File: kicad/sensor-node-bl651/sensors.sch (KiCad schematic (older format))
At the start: 11 parts, among them M1 MMC5603NJ, M2 MXC4005XC, U3 LSM303AGR

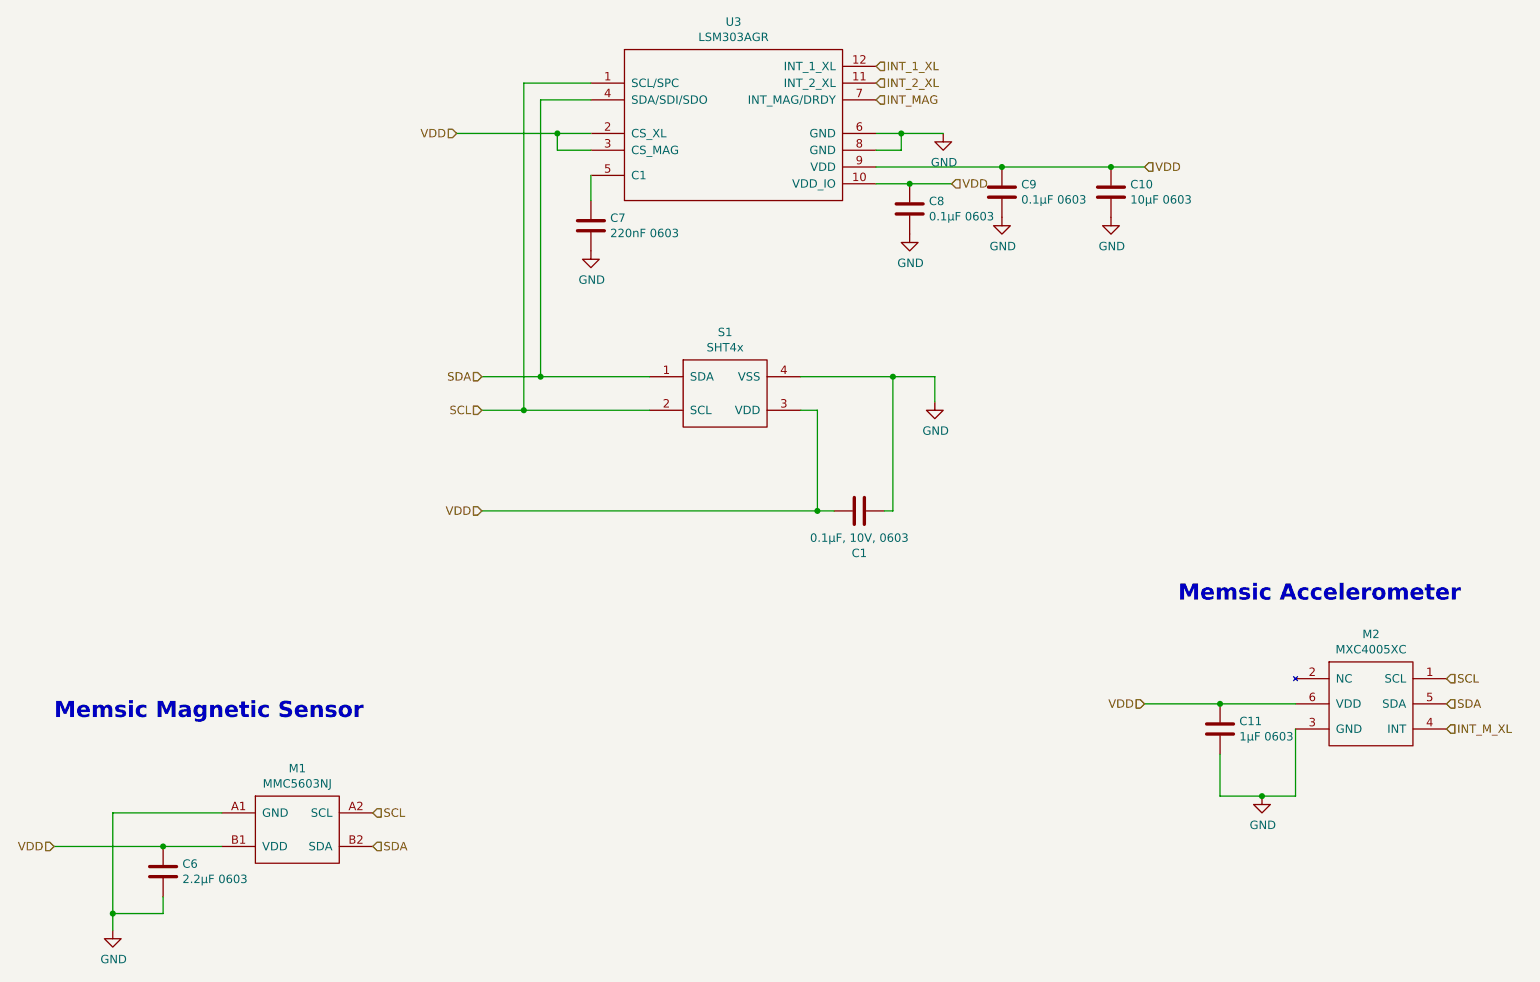
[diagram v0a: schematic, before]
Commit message: remove memsic sensors
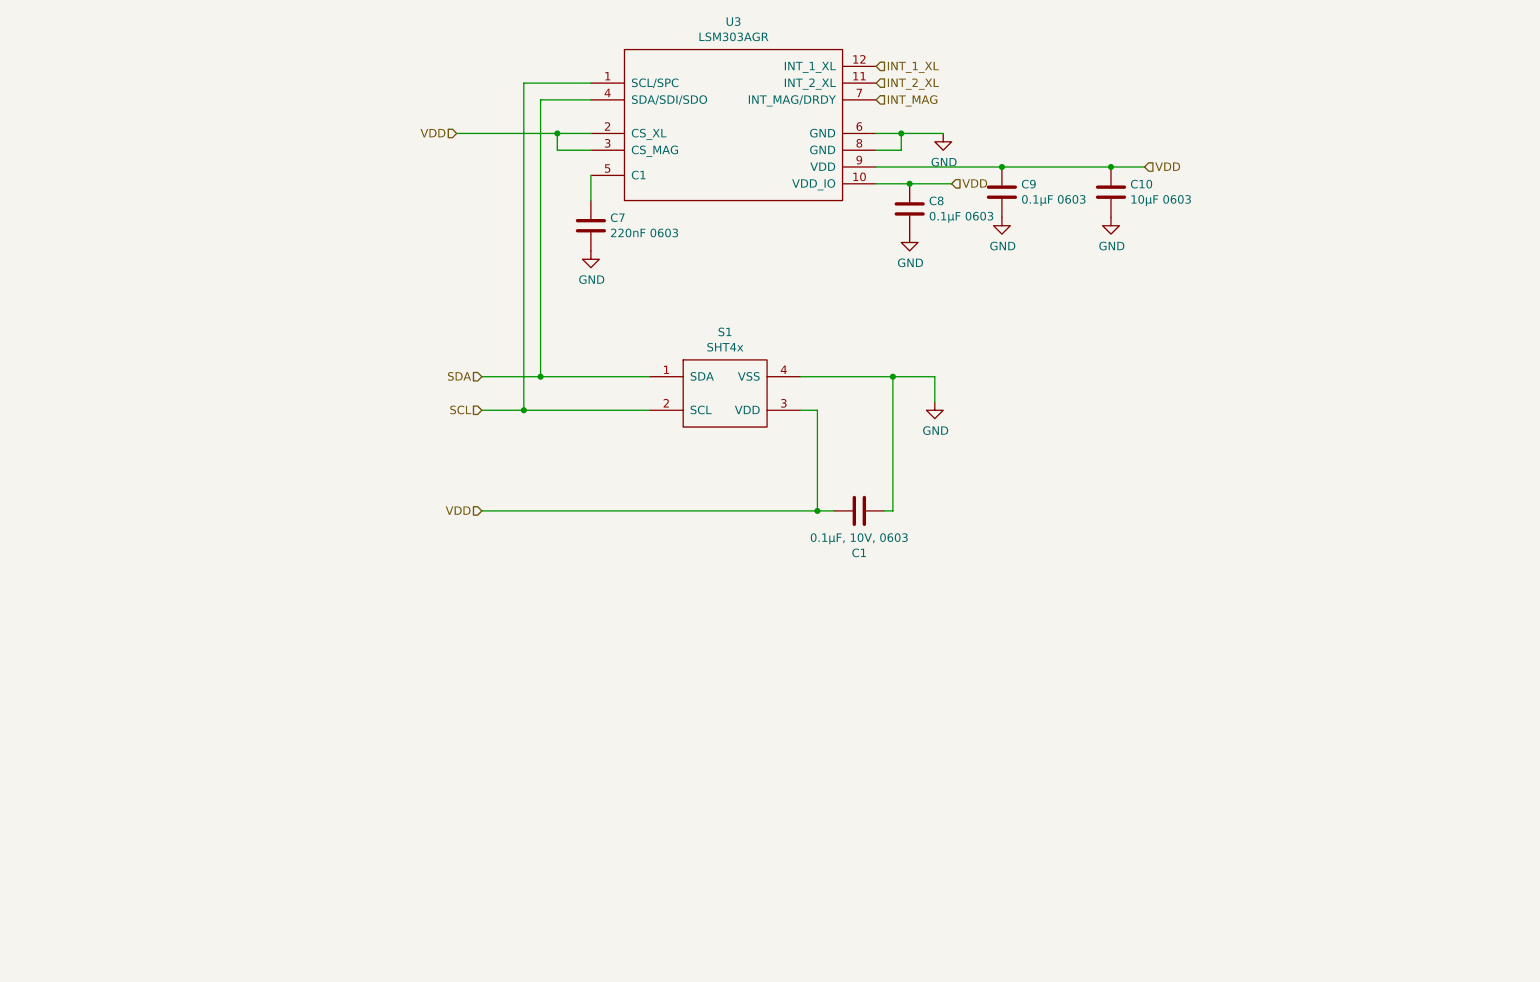
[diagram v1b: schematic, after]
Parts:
- removed C11: 1µF 0603, Capacitor_SMD:C_0603_1608Metric, symbol Device:C
- removed C6: 2.2µF 0603, Capacitor_SMD:C_0603_1608Metric, symbol Device:C
- removed M1: MMC5603NJ, HH_Memsic:MMC5603NJ, symbol HH_Memsic:MMC5603NJ
- removed M2: MXC4005XC, HH_Memsic:MXC400xXC, symbol HH_Memsic:MXC4005XC
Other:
- note removed: "Memsic Accelerometer"
- note removed: "Memsic Magnetic Sensor"
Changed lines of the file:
@@
 Wire Wire Line
 	4850 3400 5500 3400
-$Comp
-L HH_Memsic:MXC4005XC M2
-U 1 1 60BA1560
-P 9800 5350
-F 0 "M2" H 9800 5765 50  0000 C CNN
-F 1 "MXC4005XC" H 9800 5674 50  0000 C CNN
-F 2 "HH_Memsic:MXC400xXC" H 9800 5350 50  0001 C CNN
-F 3 "https://media.digikey.com/pdf/Data%20Sheets/MEMSIC%20PDFs/MXC400xXC_Rev.B_4-24-15.pdf" H 9800 5350 50  0001 C CNN
-F 4 "1267-1075-1-ND" H 9800 5350 50  0001 C CNN "Digi-Key Part Number"
-F 5 "Memsic Inc." H 9800 5350 50  0001 C CNN "Manufacturer"
-F 6 "MXC4005XC" H 9800 5350 50  0001 C CNN "Manufacturer Part Number"
-F 7 "THREE AXIS ACCELEROMETER" H 9800 5350 50  0001 C CNN "Description"
-	1    9800 5350
-	1    0    0    -1
-$EndComp
-$Comp
-L Device:C C11
-U 1 1 60BA9A12
-P 8900 5500
-F 0 "C11" H 9015 5546 50  0000 L CNN
-F 1 "1µF 0603" H 9015 5455 50  0000 L CNN
-F 2 "Capacitor_SMD:C_0603_1608Metric" H 8938 5350 50  0001 C CNN
-F 3 "~" H 8900 5500 50  0001 C CNN
-	1    8900 5500
-	1    0    0    -1
-$EndComp
-Wire Wire Line
-	8900 5350 9350 5350
-Wire Wire Line
-	9350 5500 9350 5900
-Wire Wire Line
-	9350 5900 9150 5900
-Wire Wire Line
-	8900 5900 8900 5650
-$Comp
-L power:GND #PWR010
-U 1 1 60BABF47
-P 9150 5900
-F 0 "#PWR010" H 9150 5650 50  0001 C CNN
-F 1 "GND" H 9155 5727 50  0000 C CNN
-F 2 "" H 9150 5900 50  0001 C CNN
-F 3 "" H 9150 5900 50  0001 C CNN
-	1    9150 5900
-	1    0    0    -1
-$EndComp
-Connection ~ 9150 5900
-Wire Wire Line
-	9150 5900 8900 5900
-Text HLabel 8450 5350 0    50   Input ~ 0
-VDD
-Wire Wire Line
-	8900 5350 8450 5350
-Connection ~ 8900 5350
-Text HLabel 10250 5350 2    50   Input ~ 0
-SDA
-Text HLabel 10250 5200 2    50   Input ~ 0
-SCL
-Text HLabel 10250 5500 2    50   Input ~ 0
-INT_M_XL
-Text Notes 8650 4750 0    96   ~ 19
-Memsic Accelerometer
-$Comp
-L HH_Memsic:MMC5603NJ M1
-U 1 1 60BAED17
-P 3400 6100
-F 0 "M1" H 3400 6465 50  0000 C CNN
-F 1 "MMC5603NJ" H 3400 6374 50  0000 C CNN
-F 2 "HH_Memsic:MMC5603NJ" H 3400 6100 50  0001 C CNN
-F 3 "https://media.digikey.com/pdf/Data%20Sheets/MEMSIC%20PDFs/MMC5603NJ_RevB_7-12-18.pdf" H 3400 6100 50  0001 C CNN
-F 4 "1267-MMC5603NJCT-ND" H 3400 6100 50  0001 C CNN "Digi-Key Part Number"
-F 5 "Memsic Inc." H 3400 6100 50  0001 C CNN "Manufacturer"
-F 6 "MMC5603NJ" H 3400 6100 50  0001 C CNN "Manufacturer Part Number"
-F 7 "3-AXIS AMR MAGNETIC SENSOR" H 3400 6100 50  0001 C CNN "Description"
-	1    3400 6100
-	1    0    0    -1
-$EndComp
-Text Notes 1950 5450 0    96   ~ 19
-Memsic Magnetic Sensor
-$Comp
-L Device:C C6
-U 1 1 60BB6732
-P 2600 6350
-F 0 "C6" H 2715 6396 50  0000 L CNN
-F 1 "2.2µF 0603" H 2715 6305 50  0000 L CNN
-F 2 "Capacitor_SMD:C_0603_1608Metric" H 2638 6200 50  0001 C CNN
-F 3 "~" H 2600 6350 50  0001 C CNN
-	1    2600 6350
-	1    0    0    -1
-$EndComp
-$Comp
-L power:GND #PWR09
-U 1 1 60BB7121
-P 2300 6700
-F 0 "#PWR09" H 2300 6450 50  0001 C CNN
-F 1 "GND" H 2305 6527 50  0000 C CNN
-F 2 "" H 2300 6700 50  0001 C CNN
-F 3 "" H 2300 6700 50  0001 C CNN
-	1    2300 6700
-	1    0    0    -1
-$EndComp
-Wire Wire Line
-	2300 6700 2300 6600
-Wire Wire Line
-	2300 6000 2950 6000
-Wire Wire Line
-	2600 6500 2600 6600
-Wire Wire Line
-	2600 6600 2300 6600
-Connection ~ 2300 6600
-Wire Wire Line
-	2300 6600 2300 6000
-Text HLabel 1950 6200 0    50   Input ~ 0
-VDD
-Wire Wire Line
-	1950 6200 2600 6200
-Connection ~ 2600 6200
-Wire Wire Line
-	2600 6200 2950 6200
-Text HLabel 3850 6000 2    50   Input ~ 0
-SCL
-Text HLabel 3850 6200 2    50   Input ~ 0
-SDA
 $EndSCHEMATC

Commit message: add more sensors
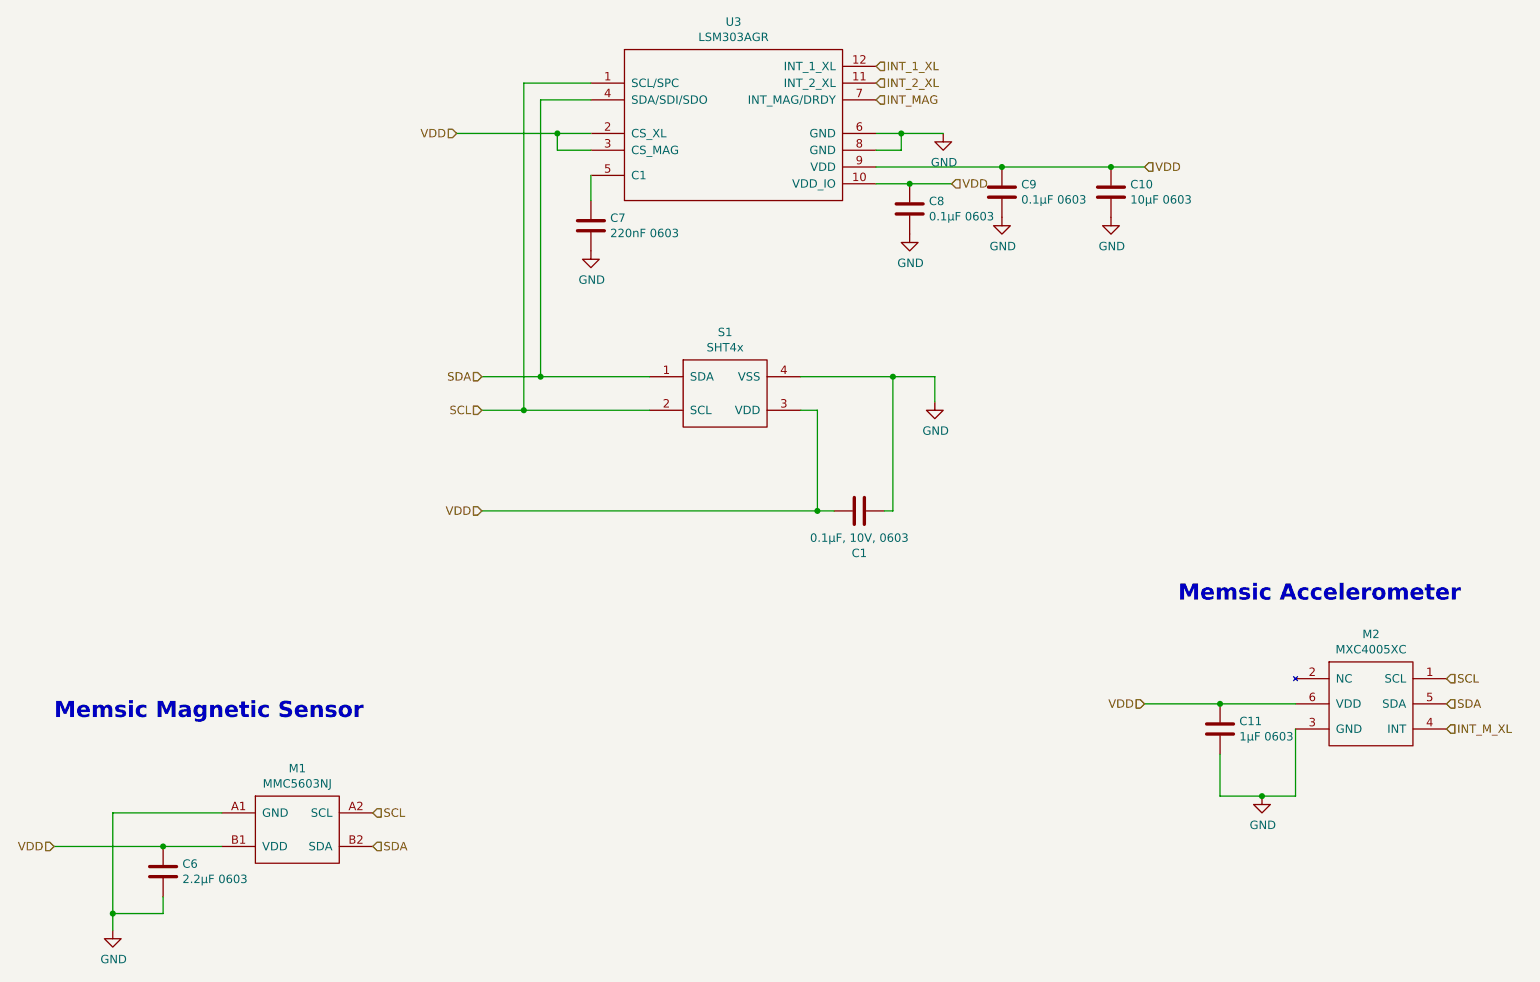
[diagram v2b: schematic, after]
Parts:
- added C11: 1µF 0603, Capacitor_SMD:C_0603_1608Metric, symbol Device:C
- added C6: 2.2µF 0603, Capacitor_SMD:C_0603_1608Metric, symbol Device:C
- added M1: MMC5603NJ, HH_Memsic:MMC5603NJ, symbol HH_Memsic:MMC5603NJ
- added M2: MXC4005XC, HH_Memsic:MXC400xXC, symbol HH_Memsic:MXC4005XC
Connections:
- net GND: now also C11.2, C6.2, M1.A1 (GND), M2.3 (GND)
- net SCL: now also M1.A2 (SCL), M2.1 (SCL)
- net SDA: now also M1.B2 (SDA), M2.5 (SDA)
- net VDD: now also C11.1, C6.1, M1.B1 (VDD), M2.6 (VDD)
- new net INT_M_XL: M2.4 (INT)
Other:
- note added: "Memsic Accelerometer"
- note added: "Memsic Magnetic Sensor"
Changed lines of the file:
@@
 Wire Wire Line
 	4850 3400 5500 3400
+$Comp
+L HH_Memsic:MXC4005XC M2
+U 1 1 60BA1560
+P 9800 5350
+F 0 "M2" H 9800 5765 50  0000 C CNN
+F 1 "MXC4005XC" H 9800 5674 50  0000 C CNN
+F 2 "HH_Memsic:MXC400xXC" H 9800 5350 50  0001 C CNN
+F 3 "https://media.digikey.com/pdf/Data%20Sheets/MEMSIC%20PDFs/MXC400xXC_Rev.B_4-24-15.pdf" H 9800 5350 50  0001 C CNN
+F 4 "1267-1075-1-ND" H 9800 5350 50  0001 C CNN "Digi-Key Part Number"
+F 5 "Memsic Inc." H 9800 5350 50  0001 C CNN "Manufacturer"
+F 6 "MXC4005XC" H 9800 5350 50  0001 C CNN "Manufacturer Part Number"
+F 7 "THREE AXIS ACCELEROMETER" H 9800 5350 50  0001 C CNN "Description"
+	1    9800 5350
+	1    0    0    -1
+$EndComp
+$Comp
+L Device:C C11
+U 1 1 60BA9A12
+P 8900 5500
+F 0 "C11" H 9015 5546 50  0000 L CNN
+F 1 "1µF 0603" H 9015 5455 50  0000 L CNN
+F 2 "Capacitor_SMD:C_0603_1608Metric" H 8938 5350 50  0001 C CNN
+F 3 "~" H 8900 5500 50  0001 C CNN
+	1    8900 5500
+	1    0    0    -1
+$EndComp
+Wire Wire Line
+	8900 5350 9350 5350
+Wire Wire Line
+	9350 5500 9350 5900
+Wire Wire Line
+	9350 5900 9150 5900
+Wire Wire Line
+	8900 5900 8900 5650
+$Comp
+L power:GND #PWR010
+U 1 1 60BABF47
+P 9150 5900
+F 0 "#PWR010" H 9150 5650 50  0001 C CNN
+F 1 "GND" H 9155 5727 50  0000 C CNN
+F 2 "" H 9150 5900 50  0001 C CNN
+F 3 "" H 9150 5900 50  0001 C CNN
+	1    9150 5900
+	1    0    0    -1
+$EndComp
+Connection ~ 9150 5900
+Wire Wire Line
+	9150 5900 8900 5900
+Text HLabel 8450 5350 0    50   Input ~ 0
+VDD
+Wire Wire Line
+	8900 5350 8450 5350
+Connection ~ 8900 5350
+Text HLabel 10250 5350 2    50   Input ~ 0
+SDA
+Text HLabel 10250 5200 2    50   Input ~ 0
+SCL
+Text HLabel 10250 5500 2    50   Input ~ 0
+INT_M_XL
+Text Notes 8650 4750 0    96   ~ 19
+Memsic Accelerometer
+$Comp
+L HH_Memsic:MMC5603NJ M1
+U 1 1 60BAED17
+P 3400 6100
+F 0 "M1" H 3400 6465 50  0000 C CNN
+F 1 "MMC5603NJ" H 3400 6374 50  0000 C CNN
+F 2 "HH_Memsic:MMC5603NJ" H 3400 6100 50  0001 C CNN
+F 3 "https://media.digikey.com/pdf/Data%20Sheets/MEMSIC%20PDFs/MMC5603NJ_RevB_7-12-18.pdf" H 3400 6100 50  0001 C CNN
+F 4 "1267-MMC5603NJCT-ND" H 3400 6100 50  0001 C CNN "Digi-Key Part Number"
+F 5 "Memsic Inc." H 3400 6100 50  0001 C CNN "Manufacturer"
+F 6 "MMC5603NJ" H 3400 6100 50  0001 C CNN "Manufacturer Part Number"
+F 7 "3-AXIS AMR MAGNETIC SENSOR" H 3400 6100 50  0001 C CNN "Description"
+	1    3400 6100
+	1    0    0    -1
+$EndComp
+Text Notes 1950 5450 0    96   ~ 19
+Memsic Magnetic Sensor
+$Comp
+L Device:C C6
+U 1 1 60BB6732
+P 2600 6350
+F 0 "C6" H 2715 6396 50  0000 L CNN
+F 1 "2.2µF 0603" H 2715 6305 50  0000 L CNN
+F 2 "Capacitor_SMD:C_0603_1608Metric" H 2638 6200 50  0001 C CNN
+F 3 "~" H 2600 6350 50  0001 C CNN
+	1    2600 6350
+	1    0    0    -1
+$EndComp
+$Comp
+L power:GND #PWR09
+U 1 1 60BB7121
+P 2300 6700
+F 0 "#PWR09" H 2300 6450 50  0001 C CNN
+F 1 "GND" H 2305 6527 50  0000 C CNN
+F 2 "" H 2300 6700 50  0001 C CNN
+F 3 "" H 2300 6700 50  0001 C CNN
+	1    2300 6700
+	1    0    0    -1
+$EndComp
+Wire Wire Line
+	2300 6700 2300 6600
+Wire Wire Line
+	2300 6000 2950 6000
+Wire Wire Line
+	2600 6500 2600 6600
+Wire Wire Line
+	2600 6600 2300 6600
+Connection ~ 2300 6600
+Wire Wire Line
+	2300 6600 2300 6000
+Text HLabel 1950 6200 0    50   Input ~ 0
+VDD
+Wire Wire Line
+	1950 6200 2600 6200
+Connection ~ 2600 6200
+Wire Wire Line
+	2600 6200 2950 6200
+Text HLabel 3850 6000 2    50   Input ~ 0
+SCL
+Text HLabel 3850 6200 2    50   Input ~ 0
+SDA
 $EndSCHEMATC
